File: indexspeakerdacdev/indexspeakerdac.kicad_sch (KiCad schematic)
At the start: 41 parts, among them IC1 MAX98360AEFB+T, IC2 MAX98360AEFB+T, IC3 W25Q16JVUXIQ_TR, J1 Conn_01x04_Pin, J2 Conn_01x11_Pin, J3 Conn_01x01_Pin, J4 Conn_01x11_Pin, J5 Conn_01x01_Pin, J6 USB_C_Plug_USB2.0, U1 RP2040, U2 MIC5317-3.3xM5, Y1 Crystal_GND24

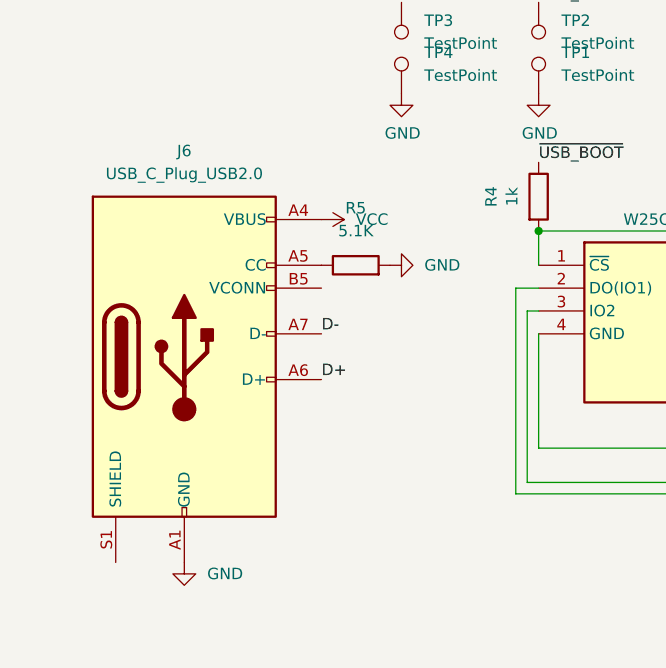
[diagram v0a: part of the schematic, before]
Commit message: Add files via upload
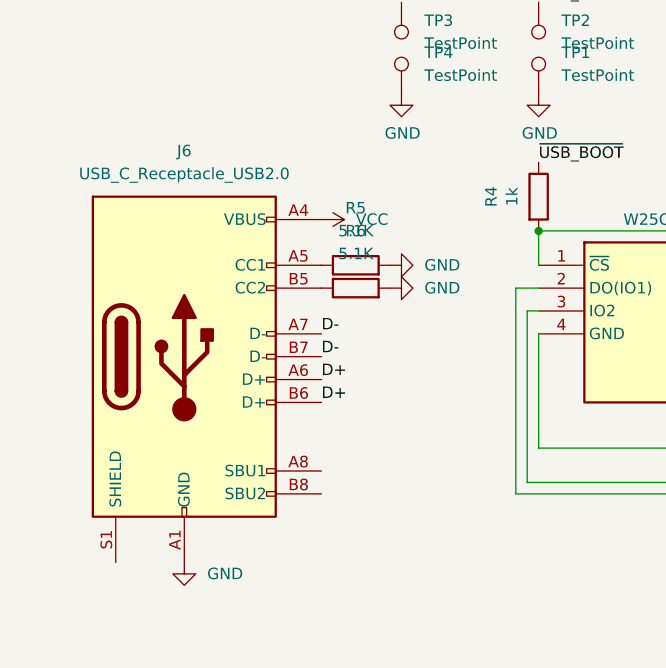
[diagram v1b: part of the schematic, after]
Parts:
- removed J6: USB_C_Plug_USB2.0, nrfmicro:USB-C-C168688, symbol Connector:USB_C_Plug_USB2.0
- added J6: USB_C_Receptacle_USB2.0, symbol Connector:USB_C_Receptacle_USB2.0
- added R6: 5.1K, Resistor_SMD:R_0201_0603Metric, symbol Device:R
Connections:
- net D+: now also J6.A6 (D+), J6.B6 (D+)
- net D-: now also J6.A7 (D-), J6.B7 (D-)
- net GND: now also J6.A1 (GND), J6.A12 (GND), J6.B1 (GND), J6.B12 (GND), R6.2
- net VCC: now also J6.A4 (VBUS), J6.A9 (VBUS), J6.B4 (VBUS), J6.B9 (VBUS)
- net at R5.1: now also J6.A5 (CC1)
- new net: J6.B5 (CC2), R6.1
